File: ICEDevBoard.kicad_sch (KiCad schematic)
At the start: 38 parts, among them J101 USB4215-03-A_REVA, Q101 BC847, U101 AP2127K-3.3, U102 AP2127K-2.5, U103 AP2127K-1.2

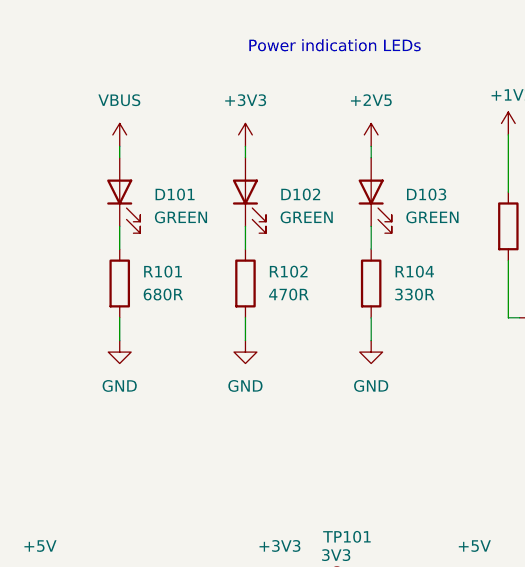
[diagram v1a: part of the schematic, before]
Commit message: Working on board layout
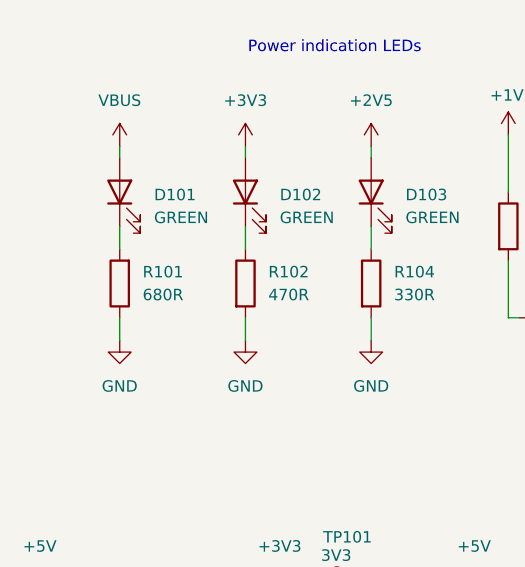
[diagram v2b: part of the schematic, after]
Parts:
- D101, D102, D103: footprint LED_SMD:LED_1210_3225Metric -> LED_SMD:LED_1206_3216Metric
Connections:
- net GND: now also R101.1; no longer R101.2
- net at D101.1 (K): now also R101.2; no longer R101.1
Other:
- moved on the sheet: R101
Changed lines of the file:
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@@
 			)
 		)
-		(property "Footprint" "LED_SMD:LED_1210_3225Metric"
+		(property "Footprint" "LED_SMD:LED_1206_3216Metric"
 			(at 30.48 114.3 0)
 			(effects
@@
 			)
 		)
-		(property "Footprint" "LED_SMD:LED_1210_3225Metric"
+		(property "Footprint" "LED_SMD:LED_1206_3216Metric"
 			(at 44.45 114.3 0)
 			(effects
@@
 	(symbol
 		(lib_id "Device:R")
-		(at 30.48 124.46 0)
+		(at 30.48 124.46 180)
 		(unit 1)
 		(exclude_from_sim no)
@@
 					(size 1.27 1.27)
 				)
-				(justify left)
+				(justify right)
 			)
 		)
@@
 					(size 1.27 1.27)
 				)
-				(justify left)
+				(justify right)
 			)
 		)
 		(property "Footprint" "Resistor_SMD:R_0805_2012Metric"
-			(at 28.702 124.46 90)
+			(at 32.258 124.46 90)
 			(effects
 				(font
@@
 			)
 		)
-		(property "Footprint" "LED_SMD:LED_1210_3225Metric"
+		(property "Footprint" "LED_SMD:LED_1206_3216Metric"
 			(at 58.42 114.3 0)
 			(effects

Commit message: More board layout
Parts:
- C108: footprint Capacitor_SMD:C_0805_2012Metric -> Capacitor_SMD:CP_Elec_4x5.3
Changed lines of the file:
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@@
 			)
 		)
-		(property "Footprint" "Capacitor_SMD:C_0805_2012Metric"
+		(property "Footprint" "Capacitor_SMD:CP_Elec_4x5.3"
 			(at 101.2952 175.26 0)
 			(effects
